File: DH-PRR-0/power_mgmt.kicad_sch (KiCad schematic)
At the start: 27 parts, among them SW2 SW_SPDT, U3 BQ25886RGE, U4 TVS0500DRV, U5 MIC5219-5.0YMM, U6 TLV75533PDRV

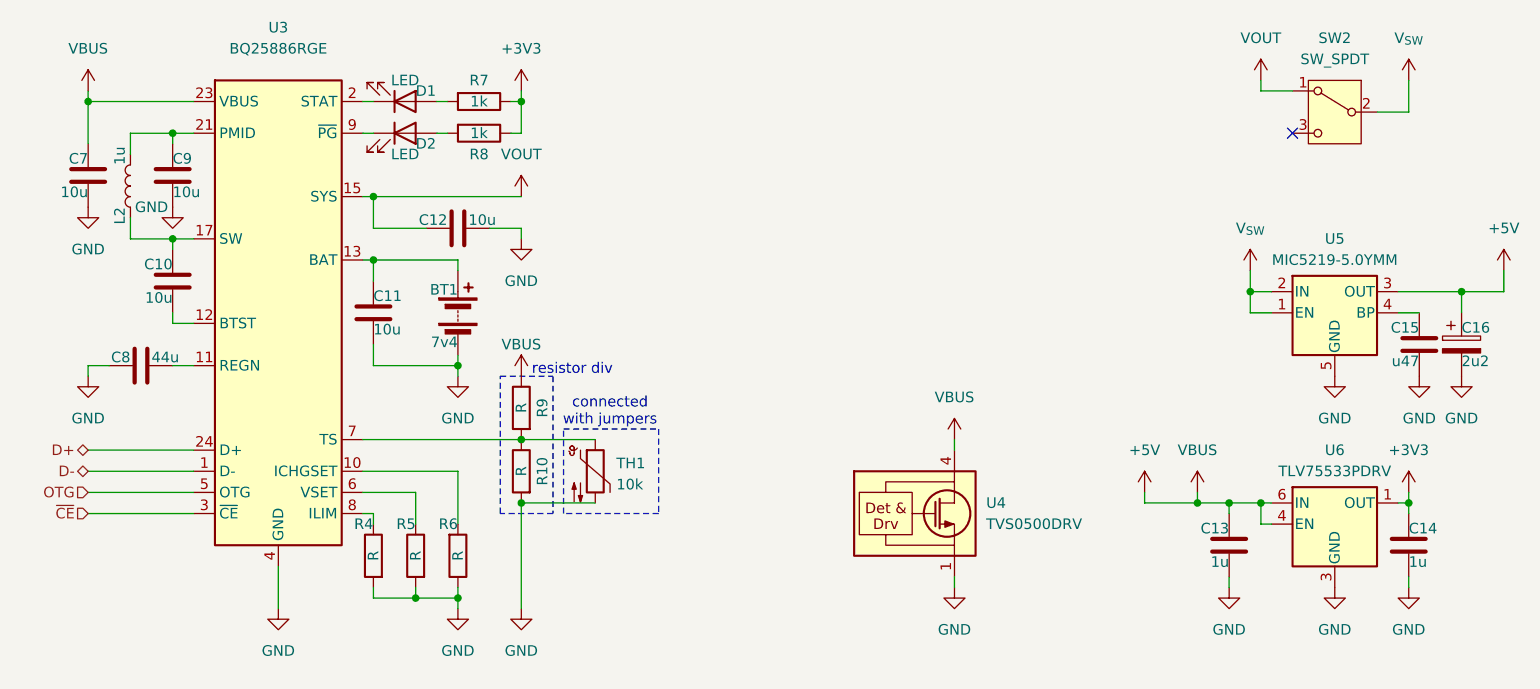
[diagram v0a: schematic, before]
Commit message: i dont remember
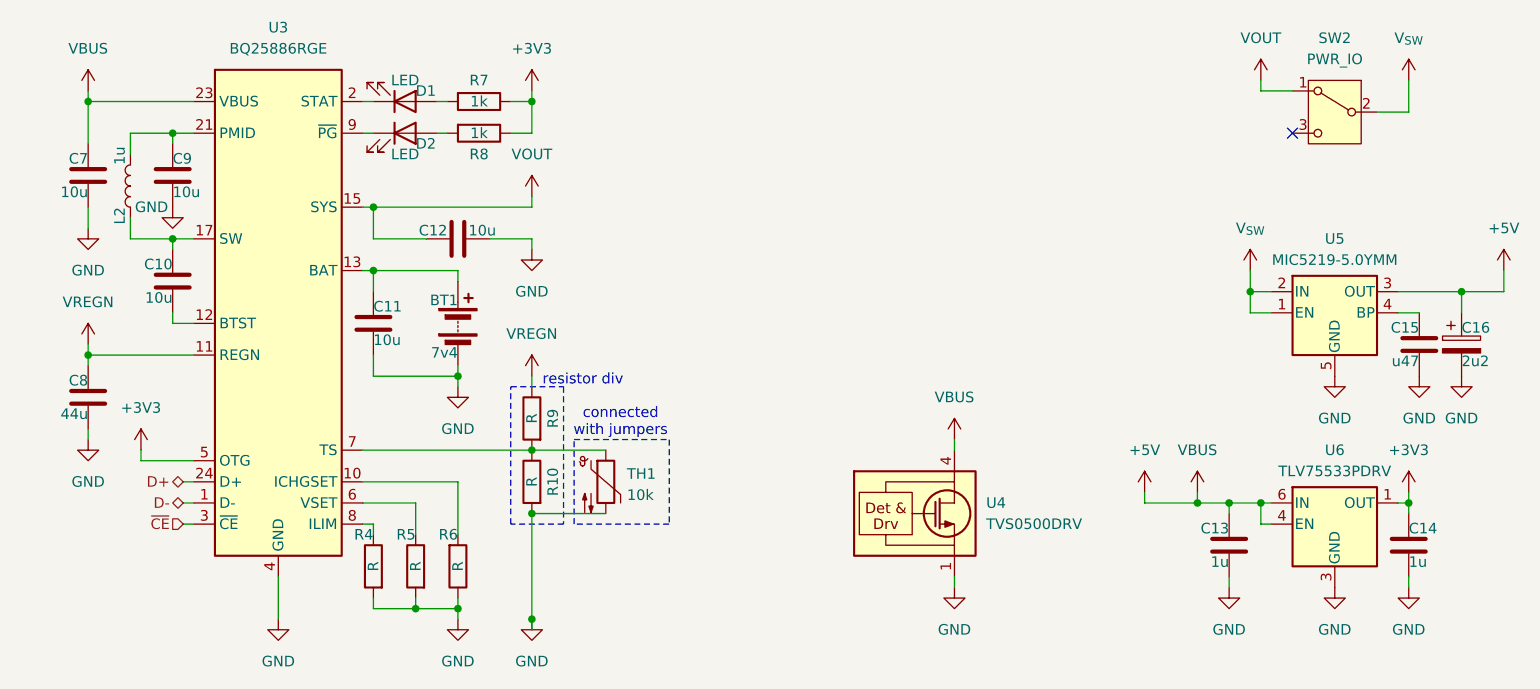
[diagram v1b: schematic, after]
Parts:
- SW2: value SW_SPDT -> PWR_IO
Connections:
- net OTG is gone; now on net +3V3: U3.5 (OTG)
- net +5V: no longer R9.1
- net GND: now also C8.2; no longer C8.1
- net VREGN: now reaches U3.11 (REGN)
- net VREGN: now also C8.1, R9.1; no longer C8.2
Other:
- moved on the sheet: BT1, C11, C12, C8, R10, R4, R5, R6, R9, TH1
